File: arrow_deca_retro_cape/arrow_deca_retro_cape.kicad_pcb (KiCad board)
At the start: 4 copper layers, 73.7 x 62 mm, 23 parts, among them J1 PMOD_A, J2 P8_Male, J3 P9_Male, U1 AS4C32M16SB-7TIN, U2 AS4C32M16SB-7TIN, U3 74LVC1G04

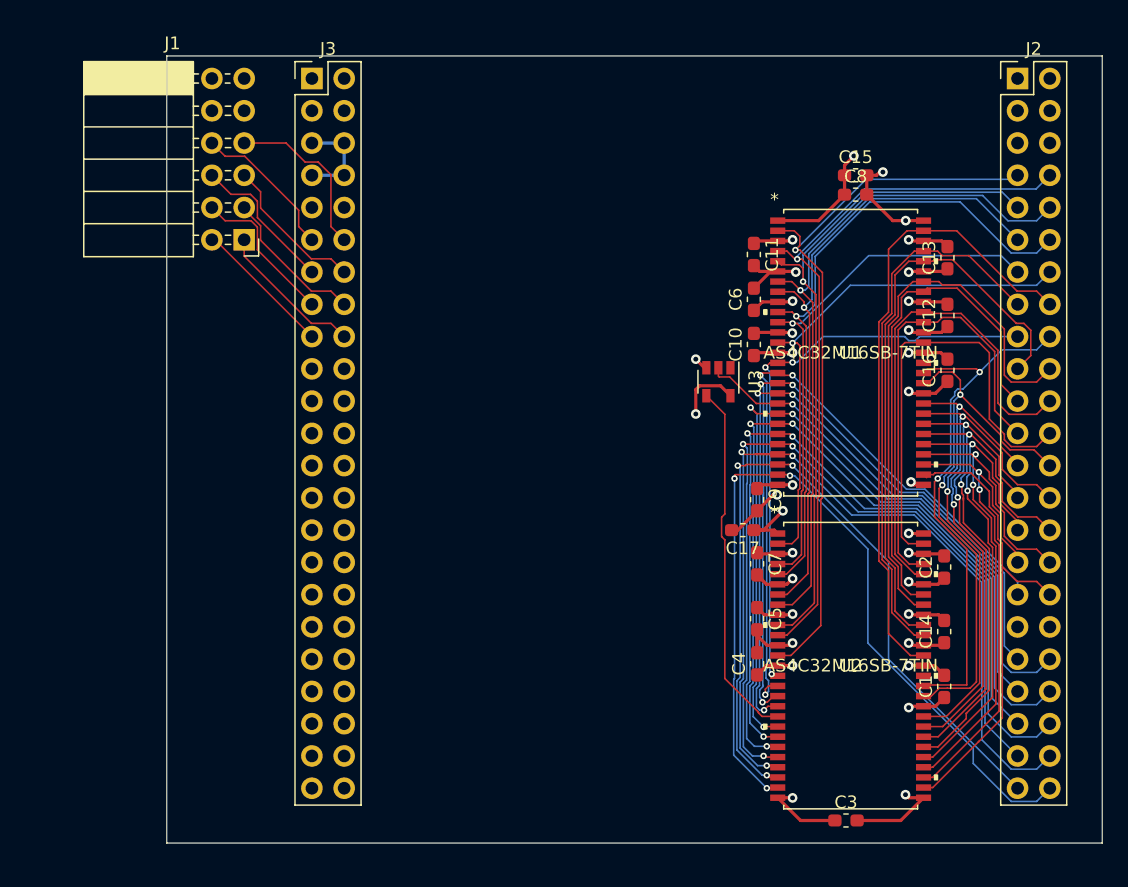
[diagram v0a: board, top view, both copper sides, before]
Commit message: Layout finished.
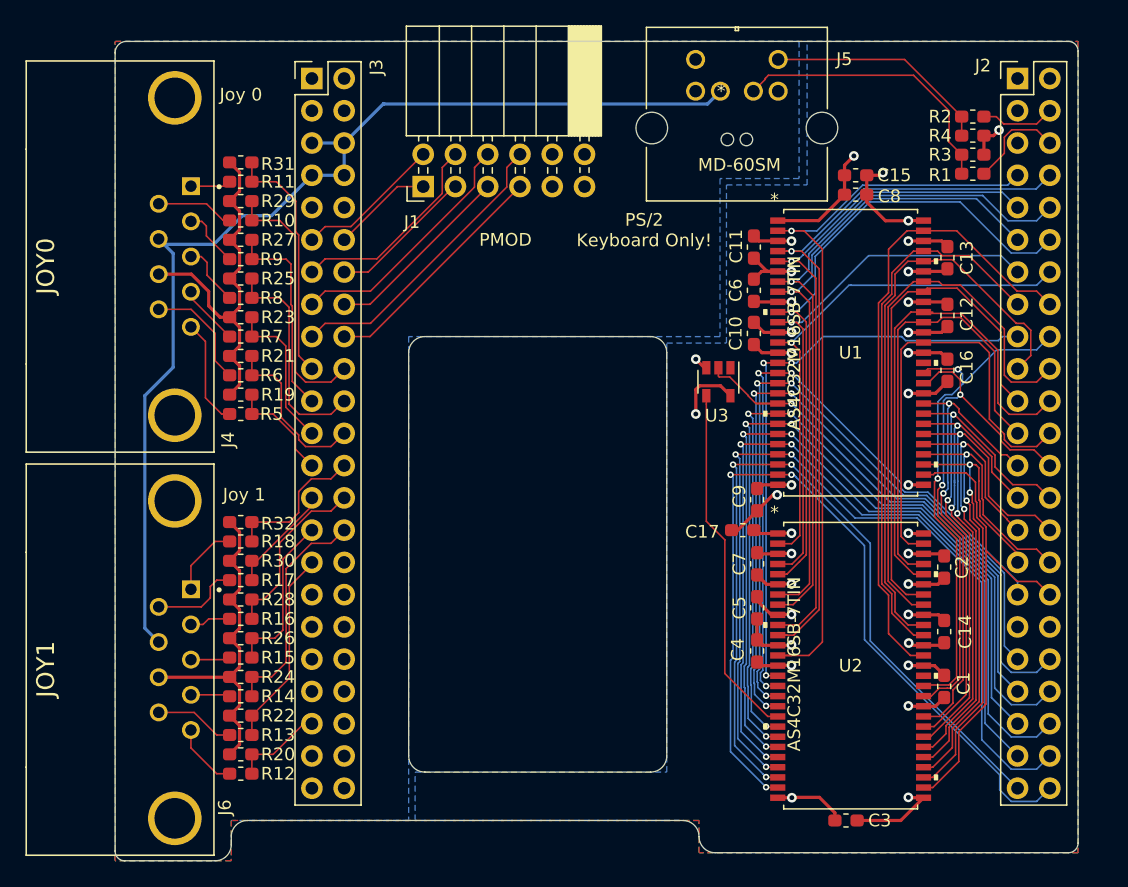
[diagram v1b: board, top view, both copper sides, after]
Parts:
- added J4: JOY0, snapeda:TE_1-1634580-2, F.Cu at (55.2, 39.4)
- added J5: MD-60SM, MD-60SM:MD-60SM, F.Cu at (100.8, 26.4)
- added J6: JOY1, snapeda:TE_1-1634580-2, F.Cu at (55.2, 71.2)
- added R1: 1K, Resistor_SMD:R_0603_1608Metric_Pad1.05x0.95mm_HandSolder, F.Cu at (118.1, 32.9)
- added R10: 2K, Resistor_SMD:R_0603_1608Metric_Pad1.05x0.95mm_HandSolder, F.Cu at (60.4, 36.6)
- added R11: 2K, Resistor_SMD:R_0603_1608Metric_Pad1.05x0.95mm_HandSolder, F.Cu at (60.4, 33.5)
- added R12: 2K, Resistor_SMD:R_0603_1608Metric_Pad1.05x0.95mm_HandSolder, F.Cu at (60.4, 80.1)
- added R13: 2K, Resistor_SMD:R_0603_1608Metric_Pad1.05x0.95mm_HandSolder, F.Cu at (60.4, 77.1)
- added R14: 2K, Resistor_SMD:R_0603_1608Metric_Pad1.05x0.95mm_HandSolder, F.Cu at (60.4, 74.0)
- added R15: 2K, Resistor_SMD:R_0603_1608Metric_Pad1.05x0.95mm_HandSolder, F.Cu at (60.4, 71.0)
- added R16: 2K, Resistor_SMD:R_0603_1608Metric_Pad1.05x0.95mm_HandSolder, F.Cu at (60.4, 67.9)
- added R17: 2K, Resistor_SMD:R_0603_1608Metric_Pad1.05x0.95mm_HandSolder, F.Cu at (60.4, 64.9)
- added R18: 2K, Resistor_SMD:R_0603_1608Metric_Pad1.05x0.95mm_HandSolder, F.Cu at (60.4, 61.8)
- added R19: 5K, Resistor_SMD:R_0603_1608Metric_Pad1.05x0.95mm_HandSolder, F.Cu at (60.4, 50.3)
- added R2: 1K, Resistor_SMD:R_0603_1608Metric_Pad1.05x0.95mm_HandSolder, F.Cu at (118.1, 28.4)
- added R20: 5K, Resistor_SMD:R_0603_1608Metric_Pad1.05x0.95mm_HandSolder, F.Cu at (60.4, 78.6)
- added R21: 5K, Resistor_SMD:R_0603_1608Metric_Pad1.05x0.95mm_HandSolder, F.Cu at (60.4, 47.2)
- added R22: 5K, Resistor_SMD:R_0603_1608Metric_Pad1.05x0.95mm_HandSolder, F.Cu at (60.4, 75.6)
- added R23: 5K, Resistor_SMD:R_0603_1608Metric_Pad1.05x0.95mm_HandSolder, F.Cu at (60.4, 44.2)
- added R24: 5K, Resistor_SMD:R_0603_1608Metric_Pad1.05x0.95mm_HandSolder, F.Cu at (60.4, 72.5)
- added R25: 5K, Resistor_SMD:R_0603_1608Metric_Pad1.05x0.95mm_HandSolder, F.Cu at (60.4, 41.1)
- added R26: 5K, Resistor_SMD:R_0603_1608Metric_Pad1.05x0.95mm_HandSolder, F.Cu at (60.4, 69.5)
- added R27: 5K, Resistor_SMD:R_0603_1608Metric_Pad1.05x0.95mm_HandSolder, F.Cu at (60.4, 38.1)
- added R28: 5K, Resistor_SMD:R_0603_1608Metric_Pad1.05x0.95mm_HandSolder, F.Cu at (60.4, 66.4)
- added R29: 5K, Resistor_SMD:R_0603_1608Metric_Pad1.05x0.95mm_HandSolder, F.Cu at (60.4, 35.1)
- added R3: 10K, Resistor_SMD:R_0603_1608Metric_Pad1.05x0.95mm_HandSolder, F.Cu at (118.1, 31.4)
- added R30: 5K, Resistor_SMD:R_0603_1608Metric_Pad1.05x0.95mm_HandSolder, F.Cu at (60.4, 63.4)
- added R31: 5K, Resistor_SMD:R_0603_1608Metric_Pad1.05x0.95mm_HandSolder, F.Cu at (60.4, 32.0)
- added R32: 5K, Resistor_SMD:R_0603_1608Metric_Pad1.05x0.95mm_HandSolder, F.Cu at (60.4, 60.3)
- added R4: 10K, Resistor_SMD:R_0603_1608Metric_Pad1.05x0.95mm_HandSolder, F.Cu at (118.1, 29.9)
- added R5: 2K, Resistor_SMD:R_0603_1608Metric_Pad1.05x0.95mm_HandSolder, F.Cu at (60.4, 51.8)
- added R6: 2K, Resistor_SMD:R_0603_1608Metric_Pad1.05x0.95mm_HandSolder, F.Cu at (60.4, 48.8)
- added R7: 2K, Resistor_SMD:R_0603_1608Metric_Pad1.05x0.95mm_HandSolder, F.Cu at (60.4, 45.7)
- added R8: 2K, Resistor_SMD:R_0603_1608Metric_Pad1.05x0.95mm_HandSolder, F.Cu at (60.4, 42.7)
- added R9: 2K, Resistor_SMD:R_0603_1608Metric_Pad1.05x0.95mm_HandSolder, F.Cu at (60.4, 39.6)
- moved J1 28.1 mm to (87.5, 33.9), turned to 270 degrees
- moved C4 1.01 mm to (101.1, 70.5)
- moved C10 0.87 mm to (100.8, 45.5)
- moved C5 0.86 mm to (101.1, 67.1)
- moved C6 0.71 mm to (100.8, 42.1)
- moved C11 0.58 mm to (100.8, 38.7)
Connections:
- J2 pad 3: Net-(J2-Pad3) -> (no net)
- J2 pad 35: Net-(J2-Pad35) -> (no net)
- J2 pad 36: Net-(J2-Pad36) -> (no net)
- J2 pad 4: Net-(J2-Pad4) -> /PS2_CLK
- J2 pad 5: Net-(J2-Pad5) -> (no net)
- J2 pad 6: Net-(J2-Pad6) -> /PS2_DATA
- J3 pad 10: /SYS_RESET_n -> (no net)
- J3 pad 11: /GPIO1_D0 -> /GPIO1_D6
- J3 pad 12: /GPIO1_D1 -> /GPIO1_D7
- J3 pad 13: /GPIO1_D2 -> /GPIO1_D4
- J3 pad 14: /GPIO1_D3 -> /GPIO1_D5
- J3 pad 15: /GPIO1_D4 -> /GPIO1_D2
- J3 pad 16: /GPIO1_D5 -> /GPIO1_D3
- J3 pad 17: /GPIO1_D6 -> /GPIO1_D0
- J3 pad 18: /GPIO1_D7 -> /GPIO1_D1
- J3 pad 19: /GPIO1_D8 -> /J0_UP
- J3 pad 20: /GPIO1_D9 -> /J0_TRIGGER
- J3 pad 21: /GPIO1_D10 -> /J0_DOWN
- J3 pad 22: /GPIO1_D11 -> /J0_LEFT
- J3 pad 23: /GPIO1_D12 -> /J0_RIGHT
- J3 pad 24: /GPIO1_D13 -> /J0_PADDLE_A
- J3 pad 25: /GPIO1_D14 -> /J0_PADDLE_B
- J3 pad 26: /GPIO1_D15 -> /J1_UP
- J3 pad 27: /GPIO1_D16 -> /J1_TRIGGER
- J3 pad 28: /GPIO1_D17 -> /J1_DOWN
- J3 pad 29: /GPIO1_D18 -> /J1_LEFT
- J3 pad 30: /GPIO1_D19 -> /J1_RIGHT
- J3 pad 31: /GPIO1_D20 -> /J1_PADDLE_A
- J3 pad 32: +1V8 -> (no net)
- J3 pad 33: /AIN6 -> (no net)
- J3 pad 34: GNDA -> (no net)
- J3 pad 35: /AIN4 -> (no net)
- J3 pad 36: /AIN5 -> (no net)
- J3 pad 37: /AIN2 -> (no net)
- J3 pad 38: /AIN3 -> (no net)
- J3 pad 39: /AIN0 -> (no net)
- J3 pad 40: /AIN1 -> (no net)
- J3 pad 41: /GPIO1_D21 -> /J1_PADDLE_B
- J3 pad 42: /GPIO1_D22 -> (no net)
- J3 pad 9: /PWR_BUT -> (no net)
- U1 pad 40: Net-(U1-Pad40) -> (no net)
- U2 pad 40: Net-(U2-Pad40) -> (no net)
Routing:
- net +5V: track 7.62 -> 87.0 mm
- net GND: track 338.8 -> 414.8 mm
- net /PS2_DATA_5V: track 0.00 -> 22.5 mm
- net /J0_TRIGGER: track 0.00 -> 20.8 mm
- net /J0_UP: track 0.00 -> 19.3 mm
- net /J1_RIGHT: track 0.00 -> 17.9 mm
- net /PS2_CLK_5V: track 0.00 -> 17.8 mm
- net /J0_LEFT: track 0.00 -> 17.5 mm
- net /J0_DOWN: track 0.00 -> 16.2 mm
- net /J1_PADDLE_A: track 0.00 -> 15.5 mm
- net /J1_DOWN: track 0.00 -> 14.0 mm
- net /J0_PADDLE_A: track 0.00 -> 13.3 mm
- net /J1_LEFT: track 0.00 -> 13.0 mm
- net /J0_RIGHT: track 0.00 -> 12.2 mm
- net /J1_UP: track 0.00 -> 11.6 mm
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- added copper zone on In2.Cu, net +3V3
- added copper zone on B.Cu, net +5V
- added copper zone on B.Cu, net GND
- added copper zone on F.Cu, net GND
- added copper zone on In1.Cu, net GND
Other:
- board size 73.7 x 62 mm -> 75.8 x 64.5 mm
- board text added: "Arrow DECA Retro Cape Tom Verbeure https://github.com/tomverbeure/arrow_deca_retro_cape"
- board text added: "Joy 0"
- board text added: "Joy 1"
- board text added: "PMOD"
- board text added: "PS/2 Keyboard Only!"
